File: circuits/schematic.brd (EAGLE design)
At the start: 79 x 41.3 mm, 42 parts, among them IC1 MEGA8-P, IC2 MAX481CPA, J1 AVR_SPI_PRG_6PTH

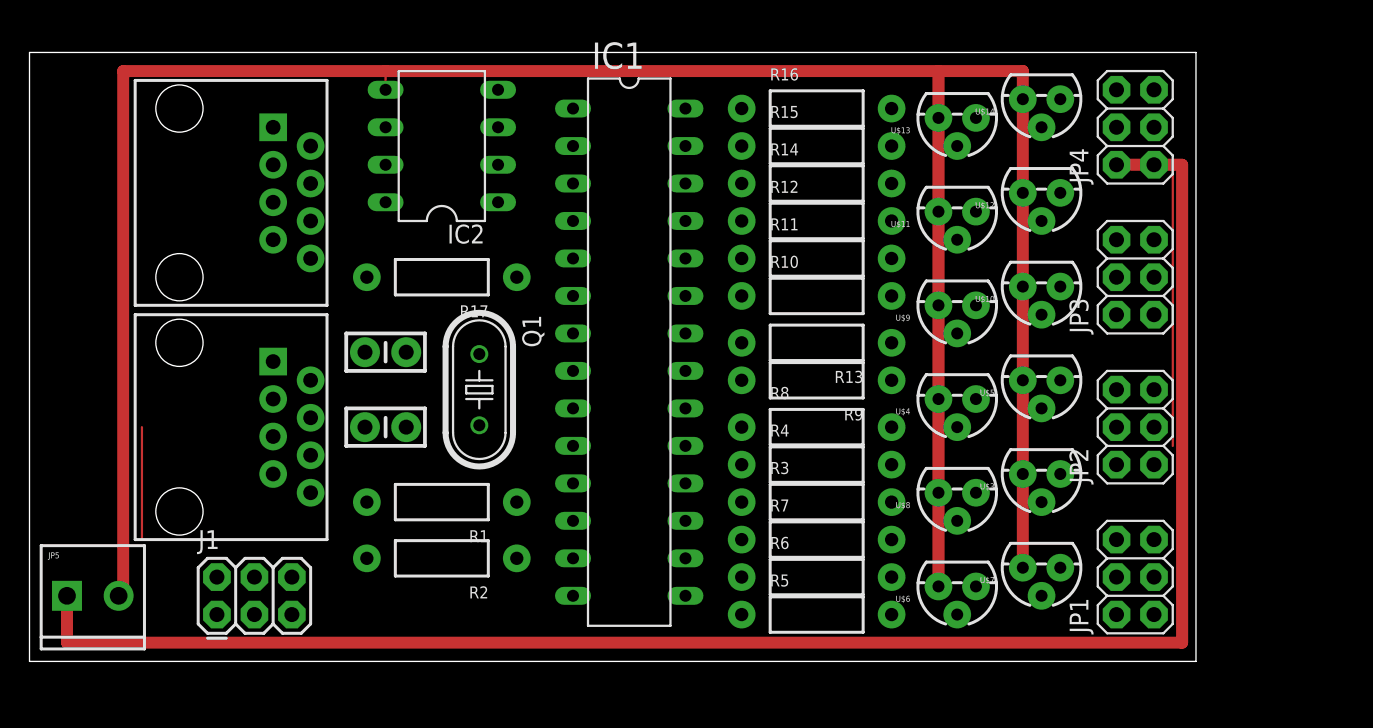
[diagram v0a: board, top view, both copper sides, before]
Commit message: Self routed version.
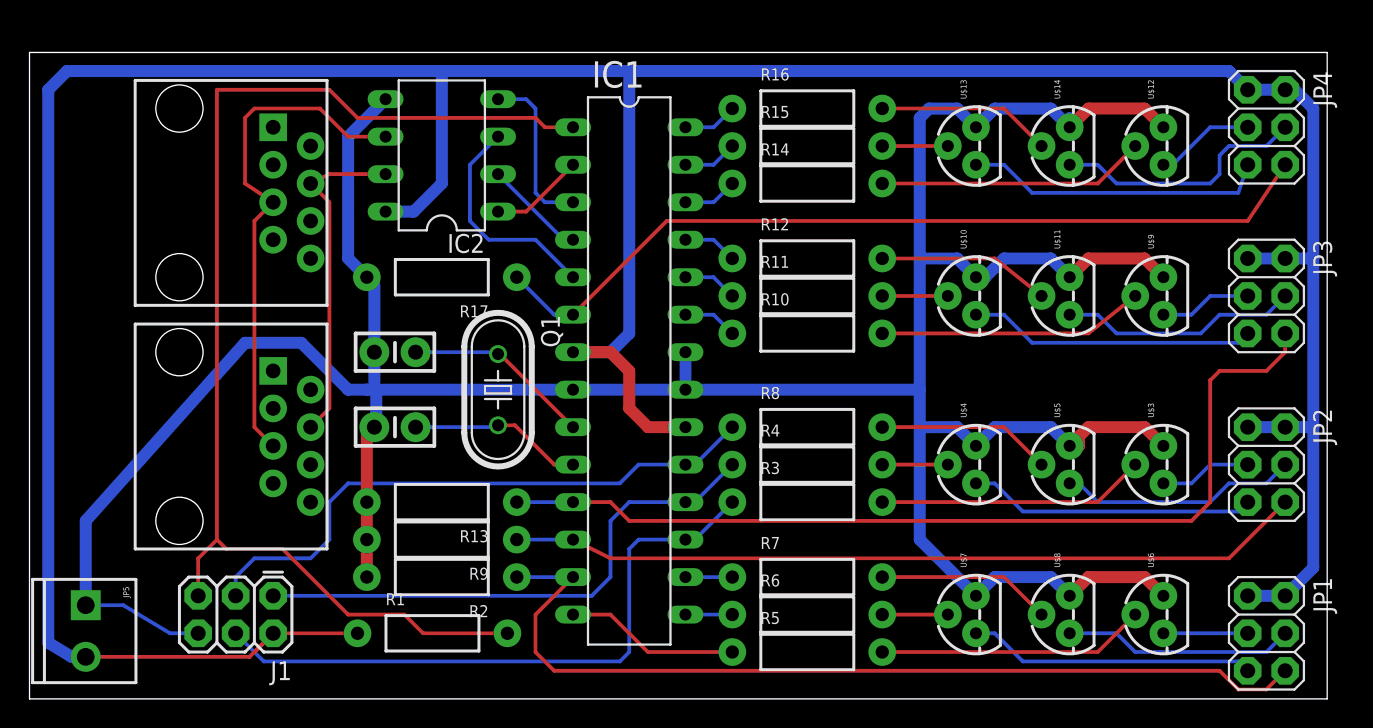
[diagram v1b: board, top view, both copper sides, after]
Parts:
- moved R13 27.6 mm to (31.8, 38.1)
- moved R9 27.6 mm to (31.8, 35.6)
- moved U$6 14.1 mm to (80.6, 30.5), turned to 90 degrees
- moved U$9 14.0 mm to (80.6, 52.1), turned to 90 degrees
- moved U$8 11.2 mm to (74.3, 30.5), turned to 90 degrees
- moved JP1 9.67 mm to (87.6, 29.2), turned to 270 degrees
- moved U$11 9.53 mm to (74.3, 52.1), turned to 90 degrees
- moved JP2 9.25 mm to (87.6, 40.6), turned to 270 degrees
- moved JP3 8.98 mm to (87.6, 52.1), turned to 270 degrees
- moved R1 8.91 mm to (31.1, 29.2), turned to 0 degrees
- moved JP4 8.89 mm to (87.6, 63.5), turned to 270 degrees
- moved U$12 8.84 mm to (80.6, 62.2), turned to 90 degrees
- moved U$3 8.28 mm to (80.6, 40.6), turned to 90 degrees
- moved U$5 6.02 mm to (74.3, 40.6), turned to 90 degrees
- moved U$7 5.46 mm to (67.9, 30.5), turned to 90 degrees
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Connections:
- net GND: now also JP5.1; no longer JP5.2
- net VCC: now also JP5.2; no longer JP5.1
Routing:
- net VCC: track 134.6 -> 239.2 mm
- net N$18: track 3.81 -> 82.3 mm
- net N$31: track 0.00 -> 63.4 mm
- net N$14: track 0.00 -> 62.3 mm
- net N$42: track 0.00 -> 57.8 mm
- net GND: track 166.7 -> 221.7 mm
- net N$21: track 0.00 -> 53.9 mm
- net N$54: track 0.00 -> 43.0 mm
- net N$26: track 0.00 -> 40.6 mm
- net N$2: track 0.00 -> 34.9 mm
- net N$55: track 7.62 -> 37.0 mm
- net N$1: track 0.00 -> 22.8 mm
- net N$52: track 0.00 -> 20.6 mm
- net N$9: track 0.00 -> 19.5 mm
- net N$40: track 0.00 -> 19.5 mm
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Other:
- board size 79 x 41.3 mm -> 87.9 x 43.8 mm
